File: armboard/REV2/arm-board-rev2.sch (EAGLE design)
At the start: 55 parts, among them J2_12V ANDERSON_POWERPOLEPP45_PCB_HO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, J2_GND ANDERSON_POWERPOLEPP45_PCB_HO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, X1 53261-06

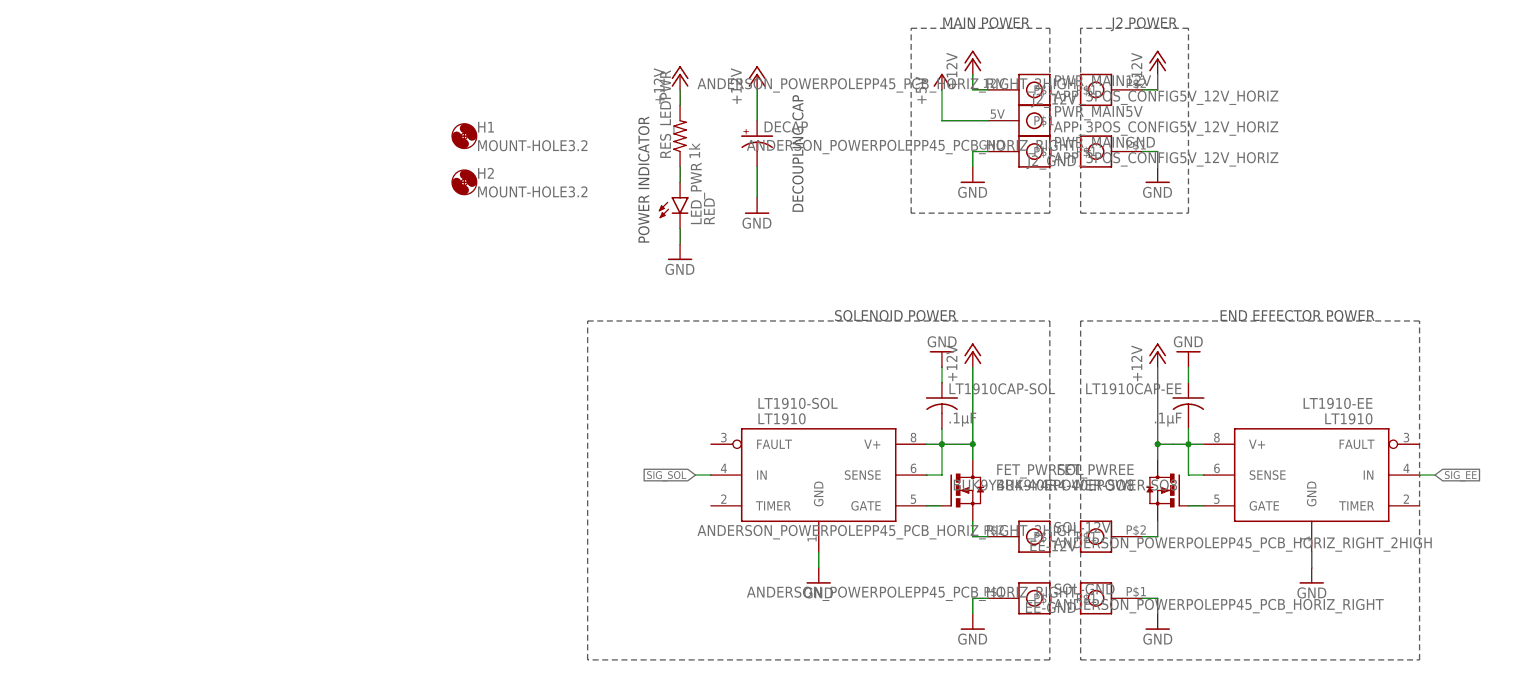
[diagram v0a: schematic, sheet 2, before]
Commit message: moved some stuff around
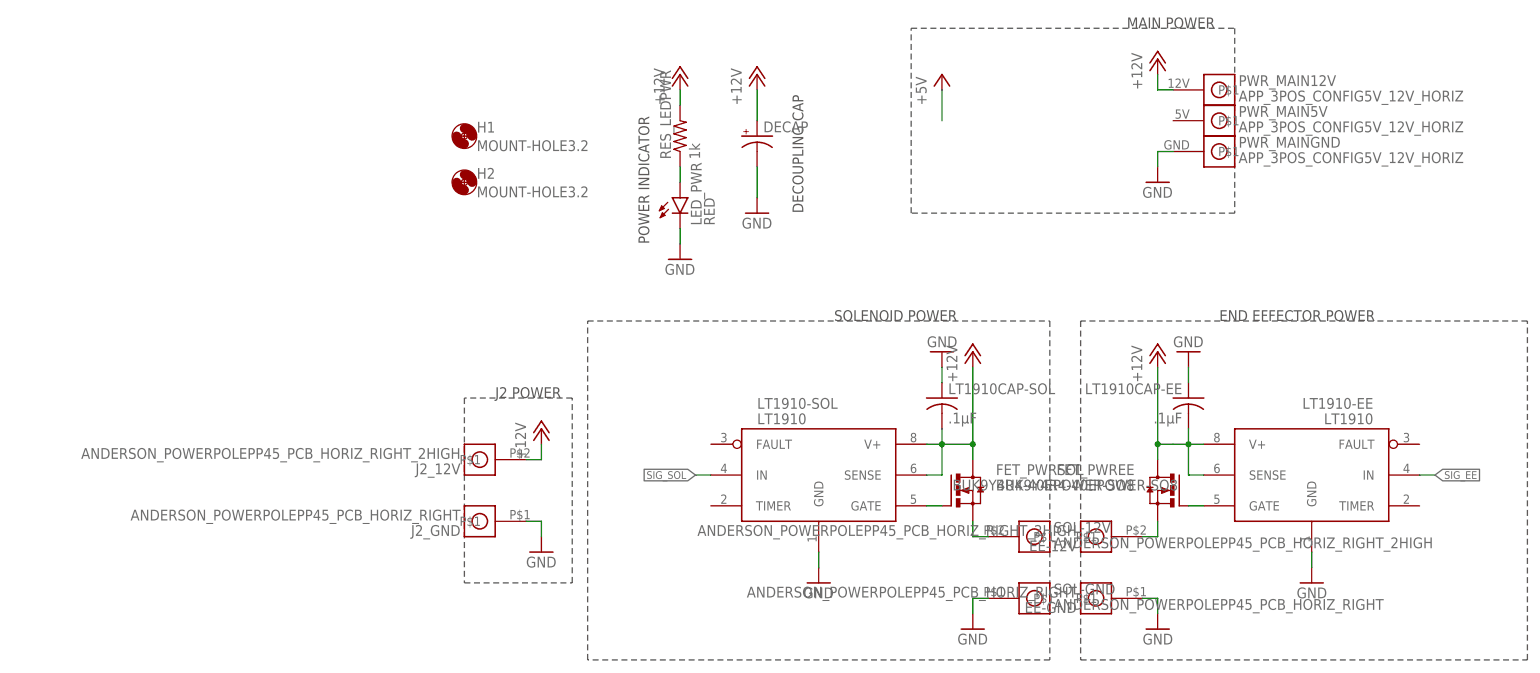
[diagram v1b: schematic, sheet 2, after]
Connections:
- net +5V: no longer PWR_MAIN5V.P$1
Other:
- moved on the sheet: J2_12V, J2_GND, PWR_MAIN12V, PWR_MAIN5V, PWR_MAINGND
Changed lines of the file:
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@@
 <part name="GND28" library="SparkFun-Aesthetics" deviceset="GND" device=""/>
 <part name="P+12" library="supply1" deviceset="+12V" device=""/>
+<part name="P+13" library="supply1" deviceset="+5V" device=""/>
 </parts>
 <sheets>
@@
 <description>Power</description>
 <plain>
-<wire x1="71.12" y1="55.88" x2="71.12" y2="25.4" width="0.1524" layer="97" style="shortdash"/>
-<wire x1="71.12" y1="25.4" x2="48.26" y2="25.4" width="0.1524" layer="97" style="shortdash"/>
+<wire x1="101.6" y1="55.88" x2="101.6" y2="25.4" width="0.1524" layer="97" style="shortdash"/>
+<wire x1="101.6" y1="25.4" x2="48.26" y2="25.4" width="0.1524" layer="97" style="shortdash"/>
 <wire x1="48.26" y1="25.4" x2="48.26" y2="55.88" width="0.1524" layer="97" style="shortdash"/>
-<wire x1="48.26" y1="55.88" x2="71.12" y2="55.88" width="0.1524" layer="97" style="shortdash"/>
-<wire x1="76.2" y1="55.88" x2="76.2" y2="25.4" width="0.1524" layer="97" style="shortdash"/>
-<wire x1="76.2" y1="25.4" x2="93.98" y2="25.4" width="0.1524" layer="97" style="shortdash"/>
-<wire x1="93.98" y1="25.4" x2="93.98" y2="55.88" width="0.1524" layer="97" style="shortdash"/>
-<wire x1="93.98" y1="55.88" x2="76.2" y2="55.88" width="0.1524" layer="97" style="shortdash"/>
-<text x="53.34" y="55.88" size="1.778" layer="97">MAIN POWER</text>
-<text x="81.28" y="55.88" size="1.778" layer="97">J2 POWER</text>
+<wire x1="48.26" y1="55.88" x2="101.6" y2="55.88" width="0.1524" layer="97" style="shortdash"/>
+<wire x1="-25.4" y1="-5.08" x2="-25.4" y2="-35.56" width="0.1524" layer="97" style="shortdash"/>
+<wire x1="-25.4" y1="-35.56" x2="-7.62" y2="-35.56" width="0.1524" layer="97" style="shortdash"/>
+<wire x1="-7.62" y1="-35.56" x2="-7.62" y2="-5.08" width="0.1524" layer="97" style="shortdash"/>
+<wire x1="-7.62" y1="-5.08" x2="-25.4" y2="-5.08" width="0.1524" layer="97" style="shortdash"/>
+<text x="83.82" y="55.88" size="1.778" layer="97">MAIN POWER</text>
+<text x="-20.32" y="-5.08" size="1.778" layer="97">J2 POWER</text>
 <wire x1="71.12" y1="7.62" x2="71.12" y2="-48.26" width="0.1524" layer="97" style="shortdash"/>
 <wire x1="71.12" y1="-48.26" x2="-5.08" y2="-48.26" width="0.1524" layer="97" style="shortdash"/>
@@
 <wire x1="-5.08" y1="7.62" x2="71.12" y2="7.62" width="0.1524" layer="97" style="shortdash"/>
 <wire x1="76.2" y1="7.62" x2="76.2" y2="-48.26" width="0.1524" layer="97" style="shortdash"/>
-<wire x1="76.2" y1="-48.26" x2="132.08" y2="-48.26" width="0.1524" layer="97" style="shortdash"/>
-<wire x1="132.08" y1="-48.26" x2="132.08" y2="7.62" width="0.1524" layer="97" style="shortdash"/>
-<wire x1="132.08" y1="7.62" x2="76.2" y2="7.62" width="0.1524" layer="97" style="shortdash"/>
+<wire x1="76.2" y1="-48.26" x2="149.86" y2="-48.26" width="0.1524" layer="97" style="shortdash"/>
+<wire x1="149.86" y1="-48.26" x2="149.86" y2="7.62" width="0.1524" layer="97" style="shortdash"/>
+<wire x1="149.86" y1="7.62" x2="76.2" y2="7.62" width="0.1524" layer="97" style="shortdash"/>
 <text x="35.56" y="7.62" size="1.778" layer="97">SOLENOID POWER</text>
 <text x="99.06" y="7.62" size="1.778" layer="97">END EFFECTOR POWER</text>
@@
 <instance part="GND2" gate="1" x="10.16" y="17.78"/>
 <instance part="P+2" gate="1" x="53.34" y="48.26"/>
-<instance part="P+3" gate="1" x="58.42" y="50.8"/>
-<instance part="GND13" gate="1" x="58.42" y="30.48"/>
+<instance part="P+3" gate="1" x="88.9" y="50.8"/>
+<instance part="GND13" gate="1" x="88.9" y="30.48"/>
 <instance part="P+4" gate="1" x="22.86" y="48.26"/>
 <instance part="DECAP" gate="G$1" x="22.86" y="38.1"/>
@@
 <instance part="P+14" gate="1" x="58.42" y="2.54"/>
 <instance part="P+15" gate="1" x="88.9" y="2.54"/>
-<instance part="P+10" gate="1" x="88.9" y="50.8"/>
-<instance part="GND9" gate="1" x="88.9" y="30.48"/>
+<instance part="P+10" gate="1" x="-12.7" y="-10.16"/>
+<instance part="GND9" gate="1" x="-12.7" y="-30.48"/>
 <instance part="GND11" gate="1" x="88.9" y="-43.18" rot="MR0"/>
 <instance part="FET_PWRSOL" gate="G$1" x="55.88" y="-20.32"/>
@@
 <instance part="SOL-12V" gate="G$1" x="68.58" y="-27.94"/>
 <instance part="EE-12V" gate="G$1" x="78.74" y="-27.94" rot="R180"/>
-<instance part="J2_GND" gate="G$1" x="78.74" y="35.56" rot="R180"/>
-<instance part="J2_12V" gate="G$1" x="78.74" y="45.72" rot="R180"/>
-<instance part="PWR_MAIN" gate="GND" x="68.58" y="35.56"/>
-<instance part="PWR_MAIN" gate="5V" x="68.58" y="40.64"/>
-<instance part="PWR_MAIN" gate="12V" x="68.58" y="45.72"/>
+<instance part="J2_GND" gate="G$1" x="-22.86" y="-25.4" rot="R180"/>
+<instance part="J2_12V" gate="G$1" x="-22.86" y="-15.24" rot="R180"/>
+<instance part="PWR_MAIN" gate="GND" x="99.06" y="35.56"/>
+<instance part="PWR_MAIN" gate="5V" x="99.06" y="40.64"/>
+<instance part="PWR_MAIN" gate="12V" x="99.06" y="45.72"/>
 <instance part="P+12" gate="1" x="10.16" y="48.26"/>
 </instances>
@@
 <net name="+12V" class="0">
 <segment>
-<wire x1="60.96" y1="45.72" x2="58.42" y2="45.72" width="0.1524" layer="91"/>
+<wire x1="91.44" y1="45.72" x2="88.9" y2="45.72" width="0.1524" layer="91"/>
 <pinref part="P+3" gate="1" pin="+12V"/>
-<wire x1="58.42" y1="45.72" x2="58.42" y2="48.26" width="0.1524" layer="91"/>
+<wire x1="88.9" y1="45.72" x2="88.9" y2="48.26" width="0.1524" layer="91"/>
 <pinref part="PWR_MAIN" gate="12V" pin="P$1"/>
 </segment>
@@
 </segment>
 <segment>
-<wire x1="86.36" y1="45.72" x2="88.9" y2="45.72" width="0.1524" layer="91"/>
+<wire x1="-15.24" y1="-15.24" x2="-12.7" y2="-15.24" width="0.1524" layer="91"/>
 <pinref part="P+10" gate="1" pin="+12V"/>
-<wire x1="88.9" y1="45.72" x2="88.9" y2="48.26" width="0.1524" layer="91"/>
+<wire x1="-12.7" y1="-15.24" x2="-12.7" y2="-12.7" width="0.1524" layer="91"/>
 <pinref part="J2_12V" gate="G$1" pin="P$1"/>
 </segment>
@@
 <net name="+5V" class="0">
 <segment>
-<wire x1="60.96" y1="40.64" x2="53.34" y2="40.64" width="0.1524" layer="91"/>
 <pinref part="P+2" gate="1" pin="+5V"/>
 <wire x1="53.34" y1="40.64" x2="53.34" y2="45.72" width="0.1524" layer="91"/>
-<pinref part="PWR_MAIN" gate="5V" pin="P$1"/>
 </segment>
 </net>
@@
 <segment>
 <pinref part="GND13" gate="1" pin="GND"/>
-<wire x1="58.42" y1="33.02" x2="58.42" y2="35.56" width="0.1524" layer="91"/>
-<wire x1="58.42" y1="35.56" x2="60.96" y2="35.56" width="0.1524" layer="91"/>
+<wire x1="88.9" y1="33.02" x2="88.9" y2="35.56" width="0.1524" layer="91"/>
+<wire x1="88.9" y1="35.56" x2="91.44" y2="35.56" width="0.1524" layer="91"/>
 <pinref part="PWR_MAIN" gate="GND" pin="P$1"/>
 </segment>
 <segment>
 <pinref part="GND9" gate="1" pin="GND"/>
-<wire x1="88.9" y1="33.02" x2="88.9" y2="35.56" width="0.1524" layer="91"/>
-<wire x1="88.9" y1="35.56" x2="86.36" y2="35.56" width="0.1524" layer="91"/>
+<wire x1="-12.7" y1="-27.94" x2="-12.7" y2="-25.4" width="0.1524" layer="91"/>
+<wire x1="-12.7" y1="-25.4" x2="-15.24" y2="-25.4" width="0.1524" layer="91"/>
 <pinref part="J2_GND" gate="G$1" pin="P$1"/>
 </segment>
@@
 <instance part="LT1910CAP-DYNA3" gate="G$1" x="213.36" y="-55.88"/>
 <instance part="GND28" gate="1" x="213.36" y="-48.26" rot="R180"/>
+<instance part="P+13" gate="1" x="119.38" y="43.18"/>
 </instances>
 <busses>
@@
 <pinref part="RES_LEDDYNASWD" gate="G$1" pin="2"/>
 <wire x1="119.38" y1="38.1" x2="119.38" y2="40.64" width="0.1524" layer="91"/>
-<label x="119.38" y="40.64" size="1.016" layer="95" rot="R90" xref="yes"/>
-</segment>
-<segment>
+<pinref part="P+13" gate="1" pin="+5V"/>
+</segment>
+<segment>
